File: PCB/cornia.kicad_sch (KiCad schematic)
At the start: 65 parts, among them SW1 SW_Push, SW10 SW_Push, SW11 SW_Push, SW12 SW_Push, SW13 SW_Push, SW14 SW_Push, SW15 SW_Push, SW16 SW_Push, SW17 SW_Push, SW18 SW_Push, SW19 SW_Push, SW2 SW_Push, SW20 SW_Push, SW21 SW_Push, SW3 SW_Push, SW4 SW_Push, SW5 SW_Push, SW6 SW_Push, SW7 SW_Push, SW8 SW_Push, SW9 SW_Push, U1 RP2040-ProMicro, U2 TRRS

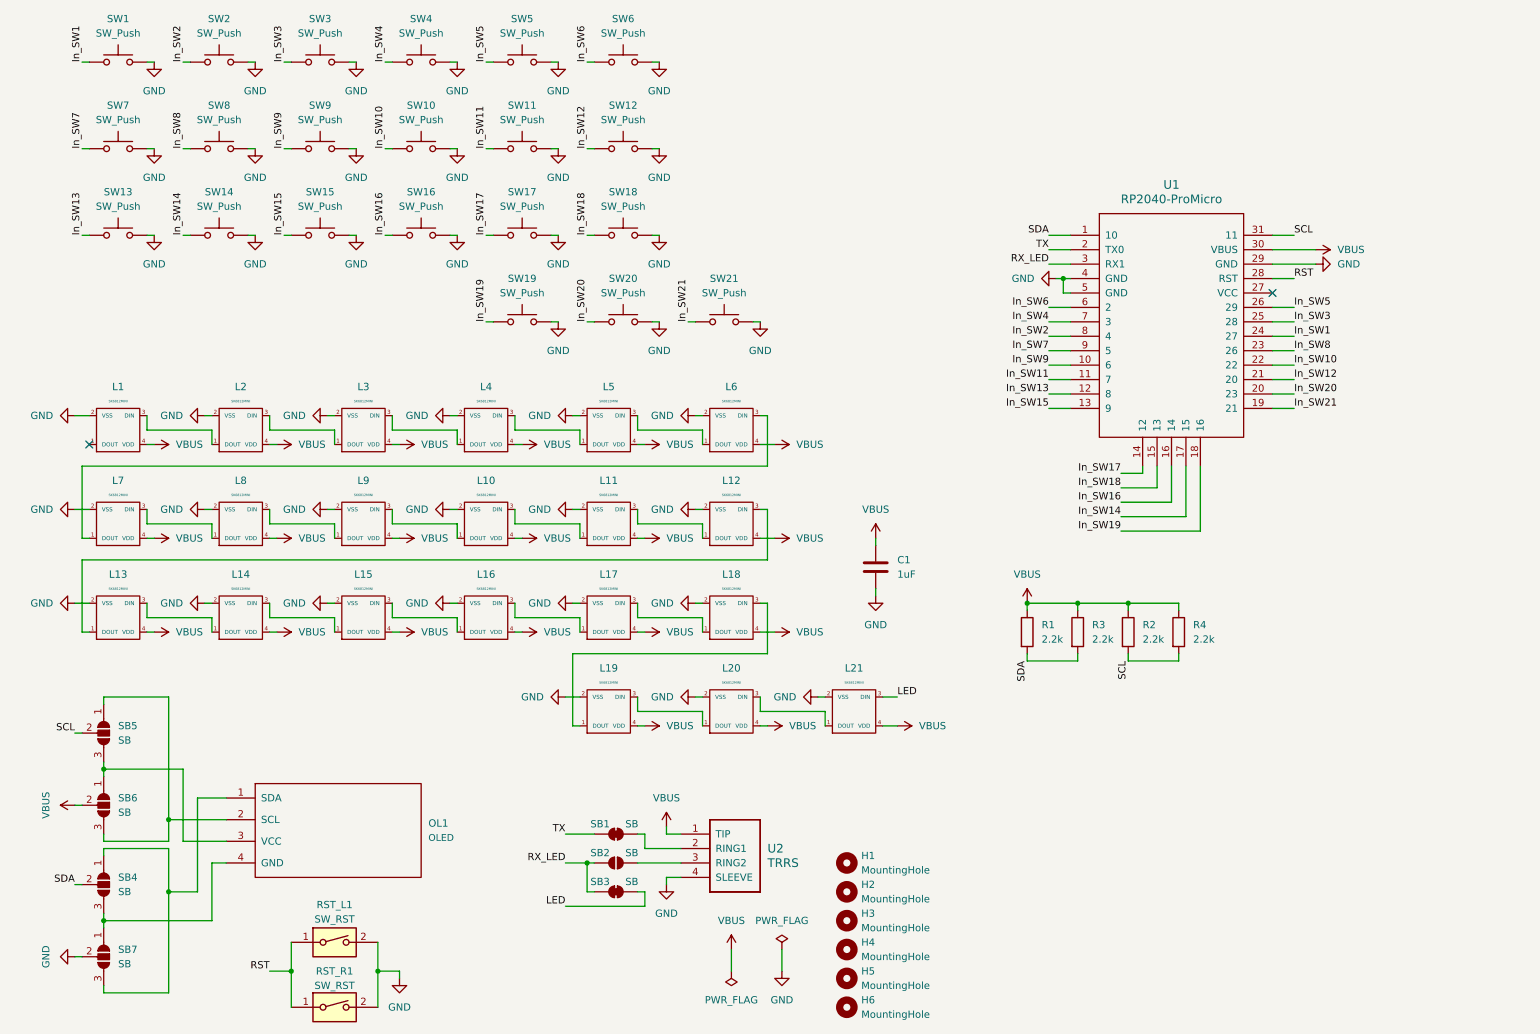
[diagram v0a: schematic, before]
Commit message: [PCB] Add handedness pin
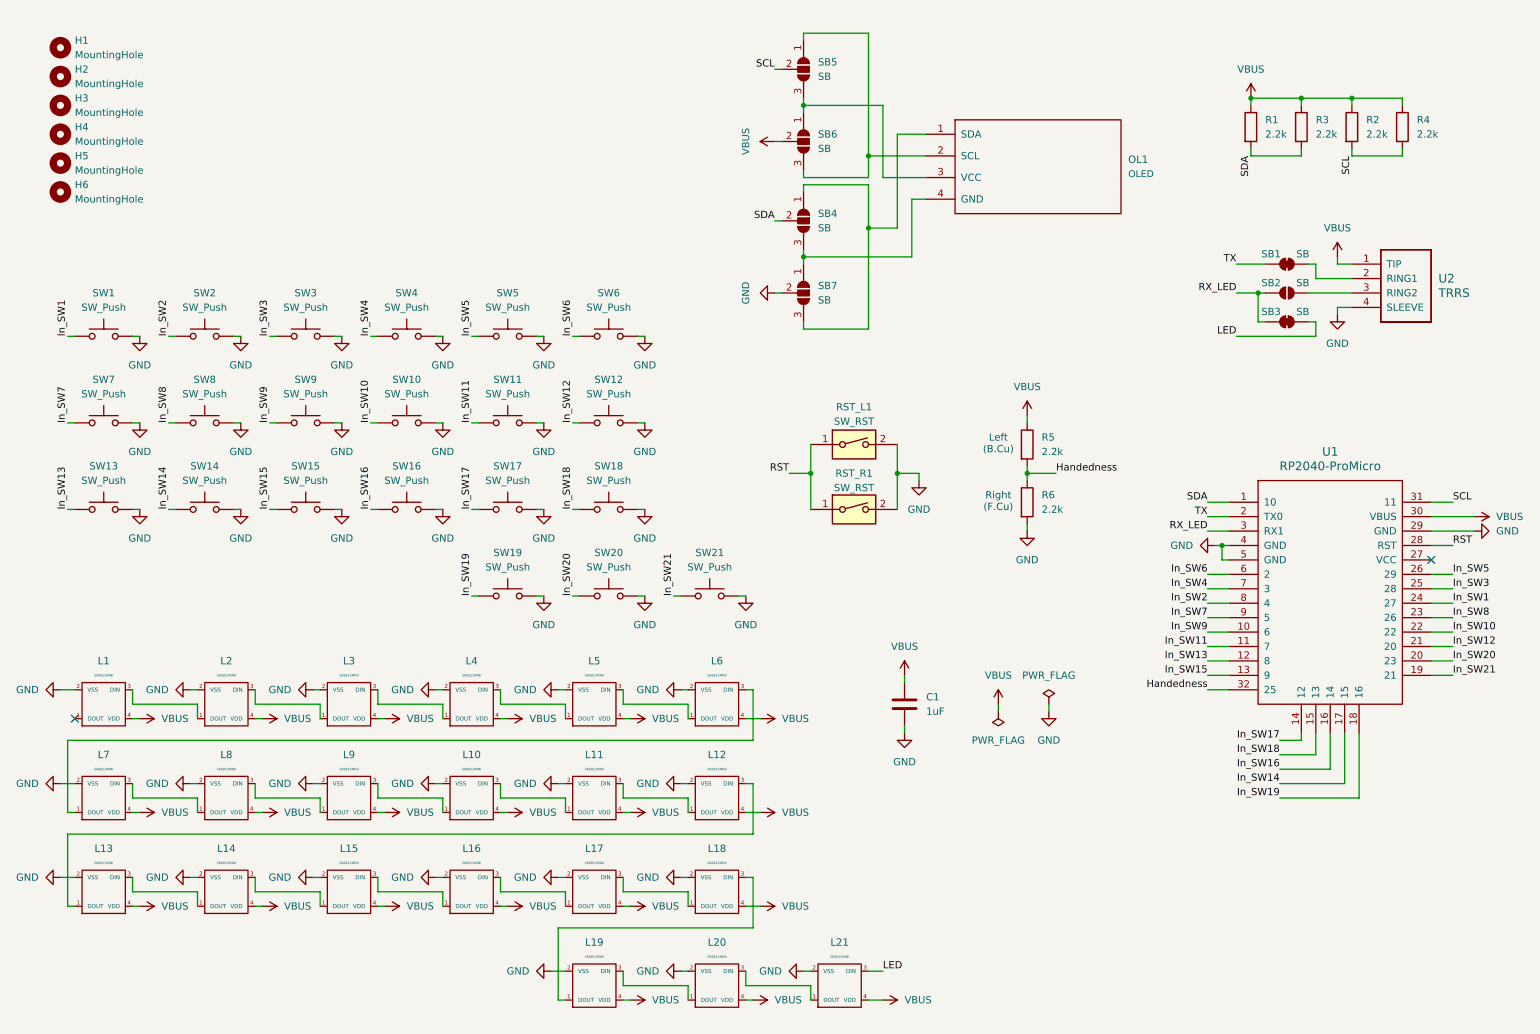
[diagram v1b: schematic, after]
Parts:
- added R5, R6: 2.2k, cornia-footprints:R_0805, symbol Device:R
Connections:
- net GND: now also R6.2
- net VBUS: now also R5.1
- new net Handedness: R5.2, R6.1, U1.32 (25)
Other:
- note added: "Left (B.Cu)"
- note added: "Right (F.Cu)"
- moved on the sheet: C1, H1, H2, H3, H4, H5, H6, L1, L10, L11, L12, L13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
